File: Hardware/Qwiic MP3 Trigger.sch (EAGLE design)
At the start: 55 parts, among them J1 MICRO-SD, J3 PTH, J7 ISP, J8 3.5mm Audio, J9 Poke-Home, U1 TPA2005D1, U2 WT2003S, U3 AP2112-3.3V, U4 ATTINY84-ARDUINO

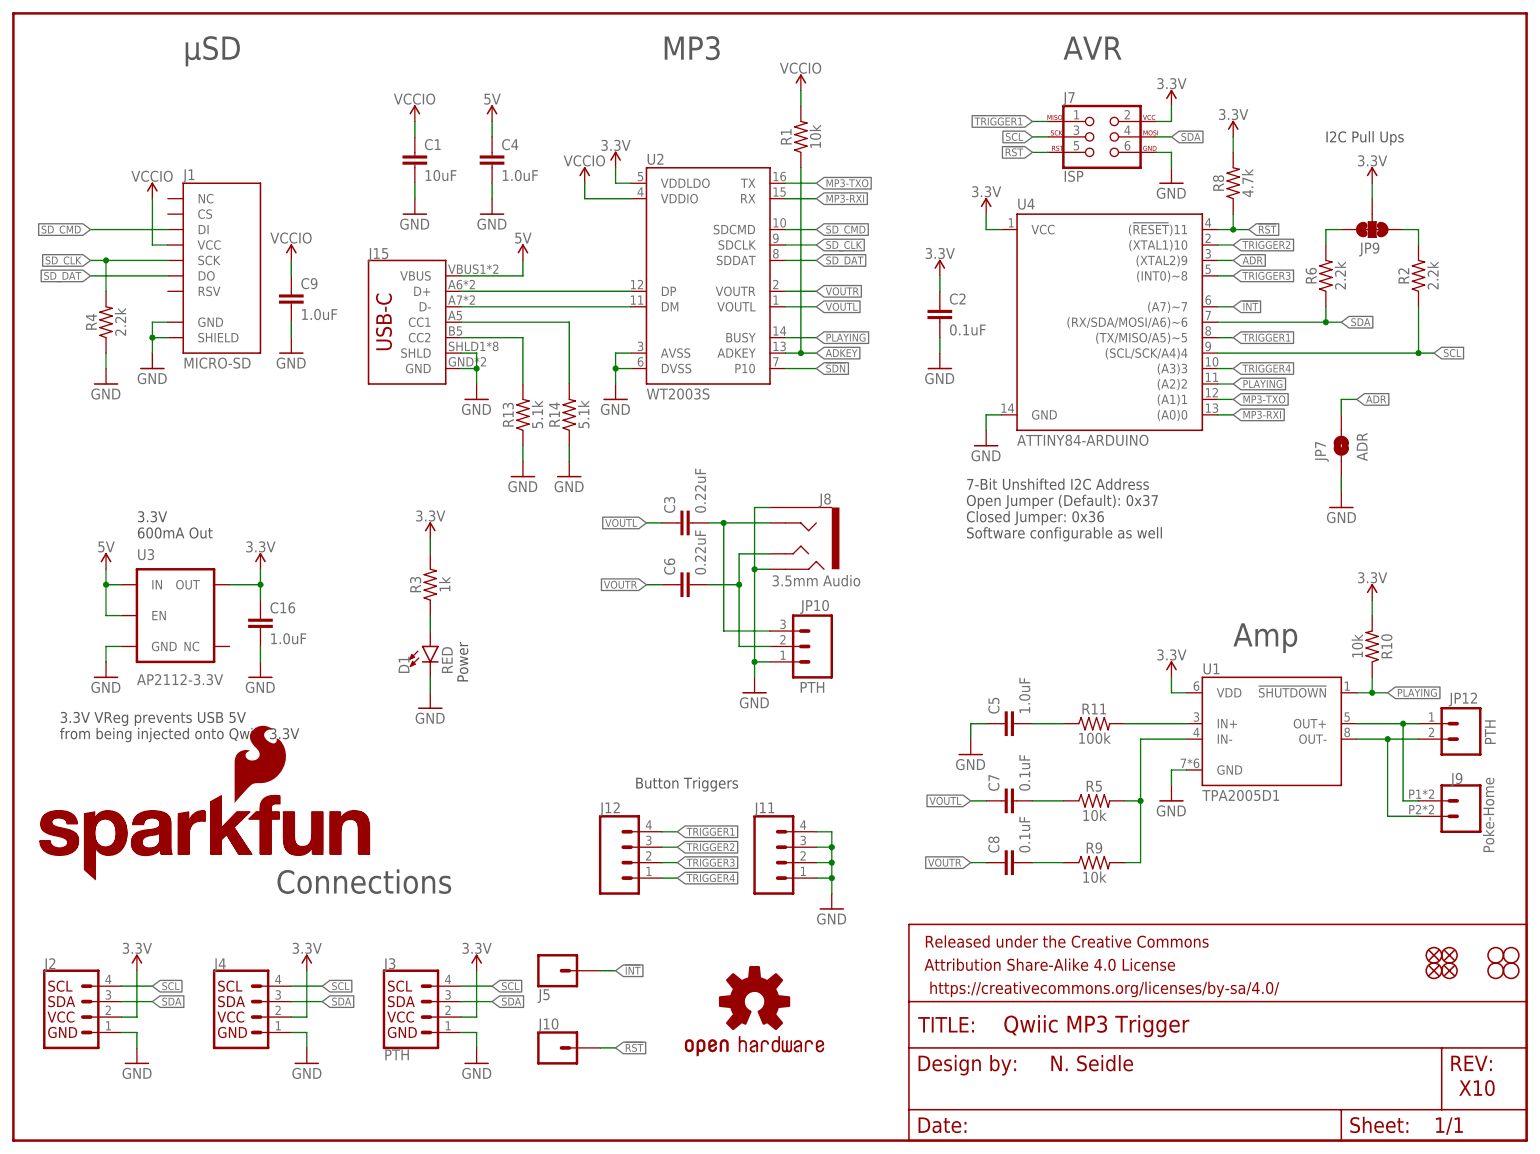
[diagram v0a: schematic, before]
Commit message: Rolling to v11 copper
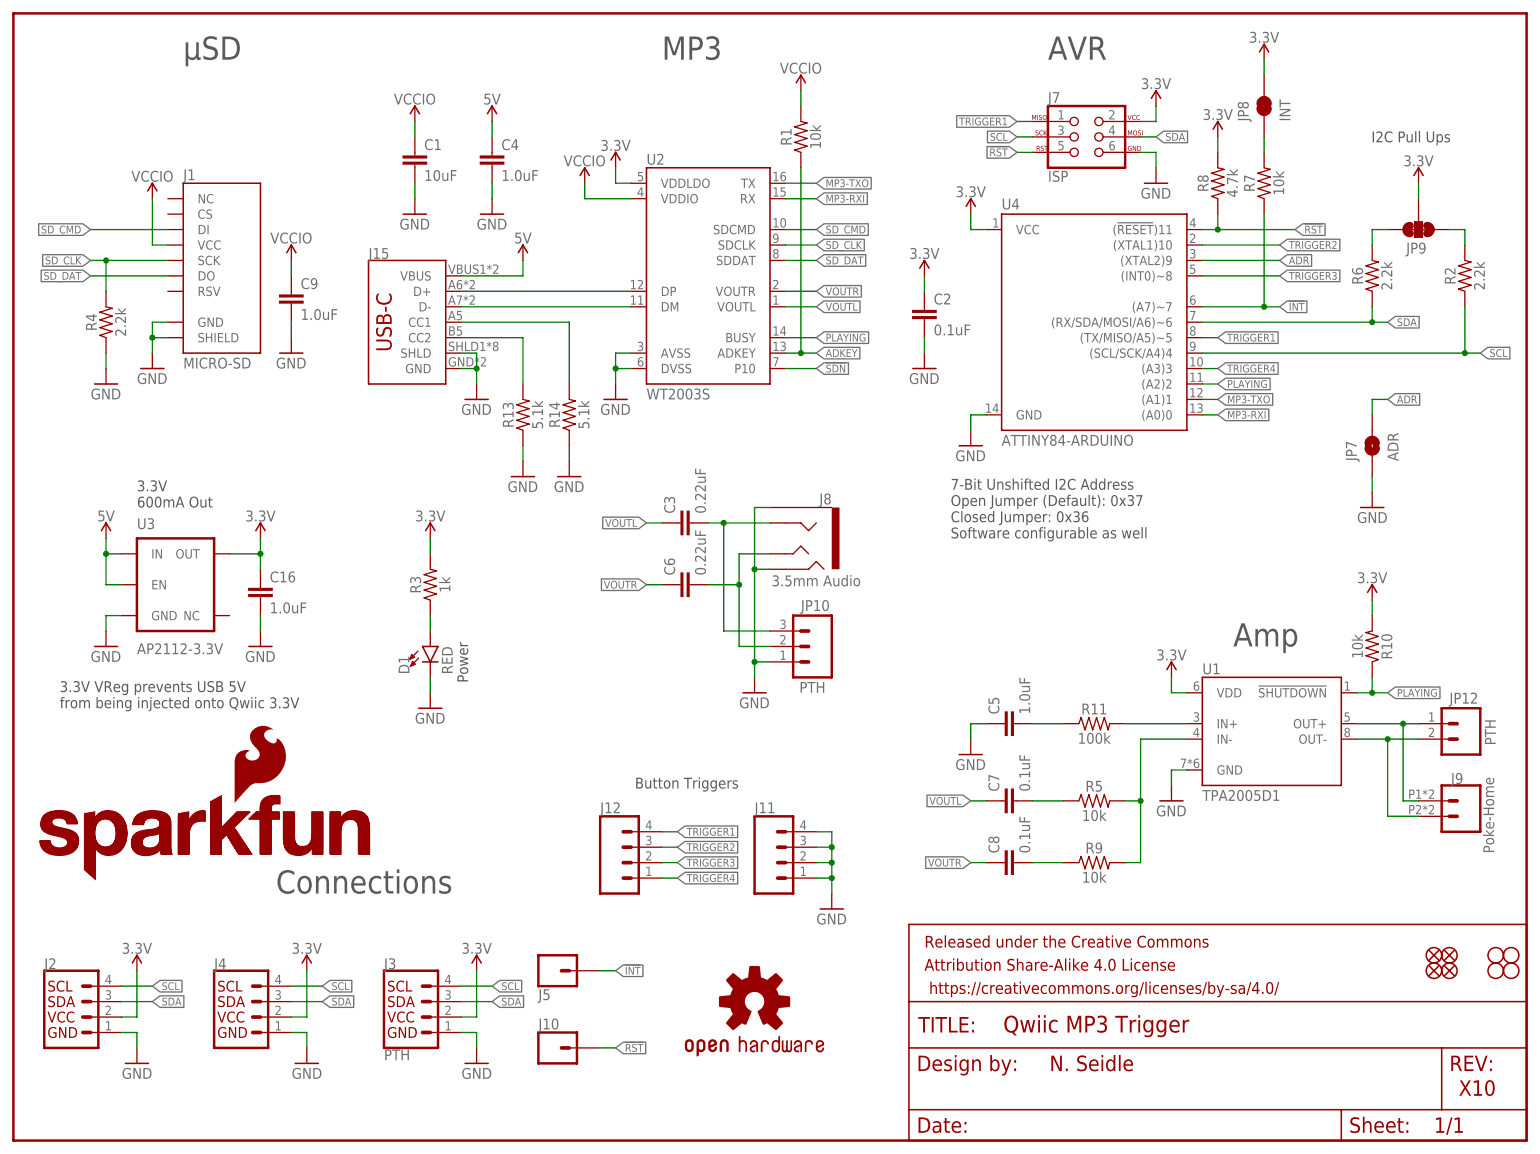
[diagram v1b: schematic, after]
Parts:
- added JP8: INT, SparkFun-Jumpers:JUMPER-SMT_2_NC_TRACE_SILK
- added R7: 10k, SparkFun-Resistors:10KOHM-0603-1/10W-1%
- JP7: device SparkFun-Jumpers:JUMPER-SMT_2_NO_NO-SILK -> SparkFun-Jumpers:JUMPER-SMT_2_NO_SILK
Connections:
- new net N$4: JP8.1, R7.2
- net !INT: now also R7.1
- net 3.3V: now also JP8.2
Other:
- moved on the sheet: C16, C2, J7, JP7, JP9, R2, R6, R8, U3, U4
